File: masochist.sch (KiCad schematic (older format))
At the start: 76 parts, among them J1 USB_C_Receptacle_USB2.0, J2 AVR-ISP-6, SW1 RESET, SW2 SW_Push, U1 ATmega328P-PU, Y1 Crystal

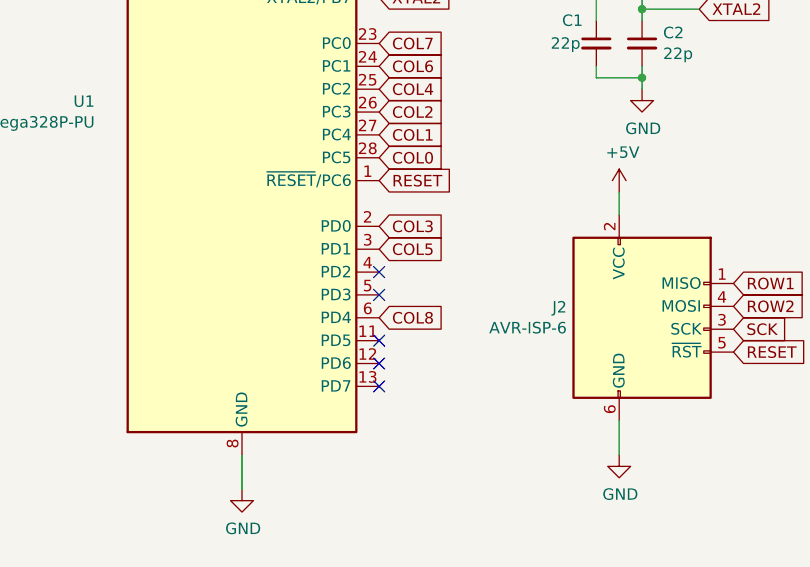
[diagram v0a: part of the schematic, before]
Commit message: Project is NOT dead, components are roughly in place
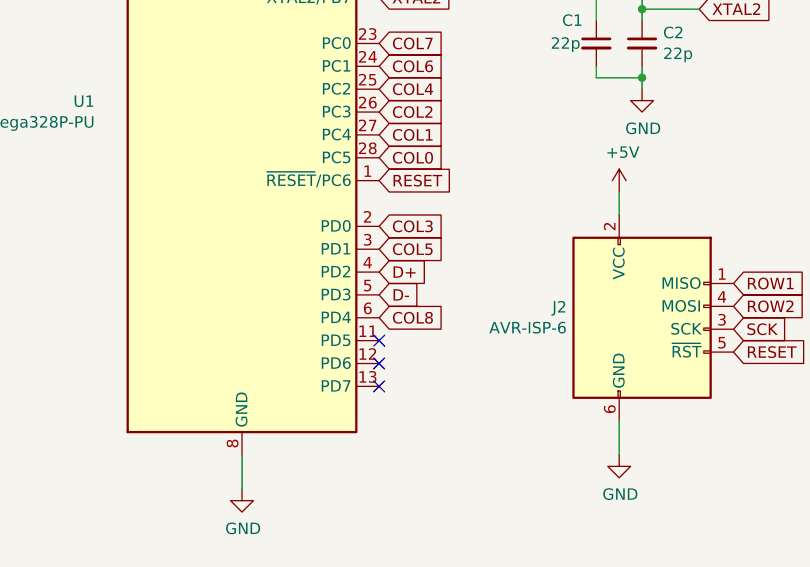
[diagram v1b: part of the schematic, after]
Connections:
- net D+: now also U1.4 (PD2)
- net D-: now also U1.5 (PD3)
- no-connect marks 8 -> 6
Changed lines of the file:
@@
 $EndDescr
-$Comp
-L MCU_Microchip_ATmega:ATmega328P-PU U1
-U 1 1 5EC3BFE1
-P 1500 2400
-F 0 "U1" H 856 2446 50  0000 R CNN
-F 1 "ATmega328P-PU" H 856 2355 50  0000 R CNN
-F 2 "Package_DIP:DIP-28_W7.62mm" H 1500 2400 50  0001 C CIN
-F 3 "http://ww1.microchip.com/downloads/en/DeviceDoc/ATmega328_P%20AVR%20MCU%20with%20picoPower%20Technology%20Data%20Sheet%2040001984A.pdf" H 1500 2400 50  0001 C CNN
-	1    1500 2400
-	1    0    0    -1
-$EndComp
 $Comp
 L power:GND #PWR0101
@@
 NoConn ~ 2100 3500
 NoConn ~ 2100 3400
-NoConn ~ 2100 3200
-NoConn ~ 2100 3100
 NoConn ~ 900  1200
+$Comp
+L MCU_Microchip_ATmega:ATmega328P-PU U1
+U 1 1 5EC3BFE1
+P 1500 2400
+F 0 "U1" H 856 2446 50  0000 R CNN
+F 1 "ATmega328P-PU" H 856 2355 50  0000 R CNN
+F 2 "Package_DIP:DIP-28_W7.62mm" H 1500 2400 50  0001 C CIN
+F 3 "http://ww1.microchip.com/downloads/en/DeviceDoc/ATmega328_P%20AVR%20MCU%20with%20picoPower%20Technology%20Data%20Sheet%2040001984A.pdf" H 1500 2400 50  0001 C CNN
+	1    1500 2400
+	1    0    0    -1
+$EndComp
+Text GLabel 2100 3100 2    50   Input ~ 0
+D+
+Text GLabel 2100 3200 2    50   Input ~ 0
+D-
 $EndSCHEMATC
